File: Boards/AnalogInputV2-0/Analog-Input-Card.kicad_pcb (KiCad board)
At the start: 2 copper layers, 80 x 72 mm, 63 parts, among them IC1 PIC32MM0064GPM028, P1 6x1 2.54, P1 usb1.1, P2 Inputs, P3 Earth, Q1 AO3407A, Q2 NX7002AK, Q3 NX7002AK, Q4 NX7002AK, U1 ST485EC, U2 MCP3428, U3 AP2114H, X1 8MHz

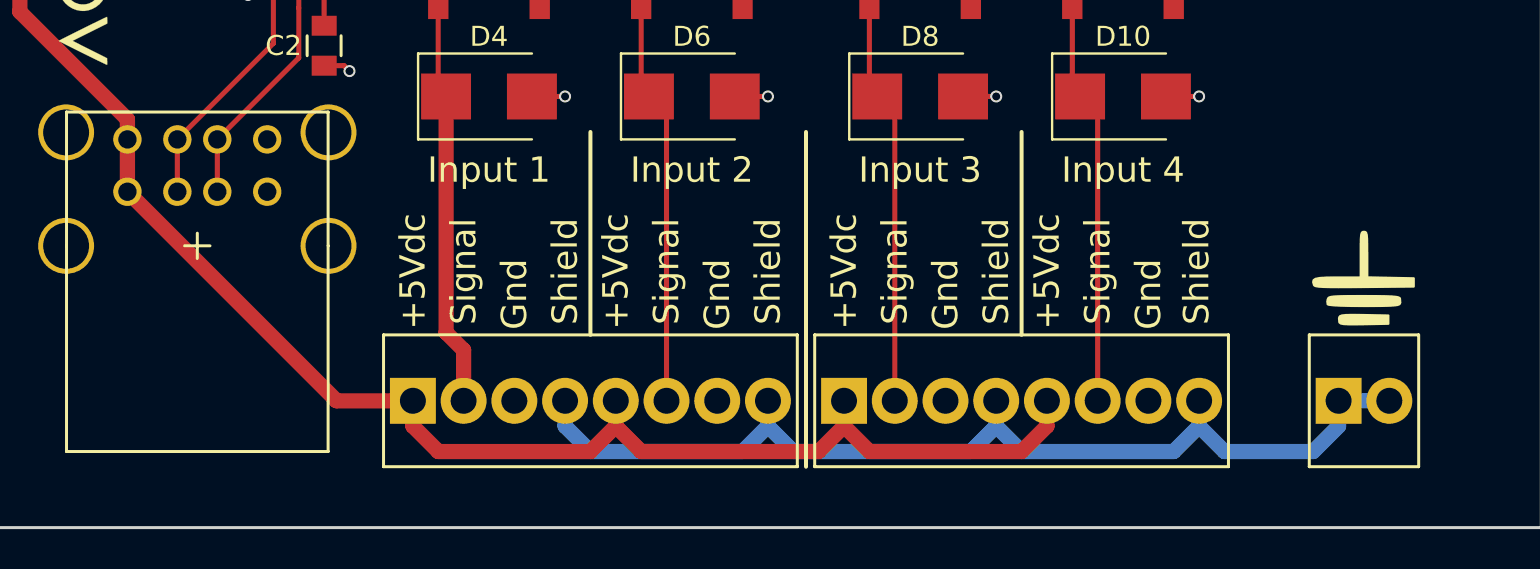
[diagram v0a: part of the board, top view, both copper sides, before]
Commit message: more work on uniformity between boards
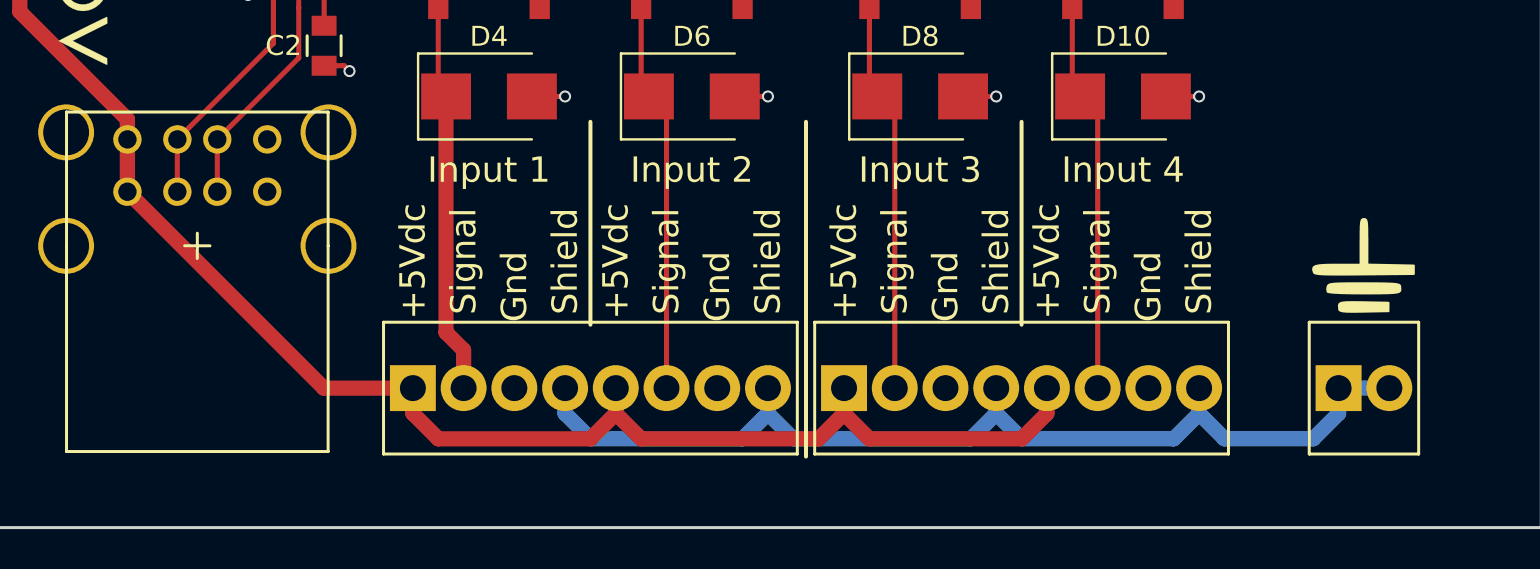
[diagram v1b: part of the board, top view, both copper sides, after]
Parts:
- moved P2 0.64 mm to (43.2, -6.99)
- moved P3 0.64 mm to (71.1, -6.99)
- moved G*** 0.63 mm to (71.1, -12.1)
